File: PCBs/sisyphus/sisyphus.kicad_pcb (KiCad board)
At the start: 2 copper layers, 60 x 39.5 mm, 65 parts, among them J1 USB_C_Receptacle_USB2.0_14P, J2 AUX USB, J3 Conn_01x02, J4 Speaker, J5 SWD, J6 RGB_CONN, J7 Keyboard, J8 Light sensor, J9 Battery, U1 NCP1117-3.3_SOT223, U2 USBLC6-2P6, U3 W25Q128JVS, U4 MAX98357A, U5 RP2040, U7 BQ25619, Y1 ABM8-272-T3

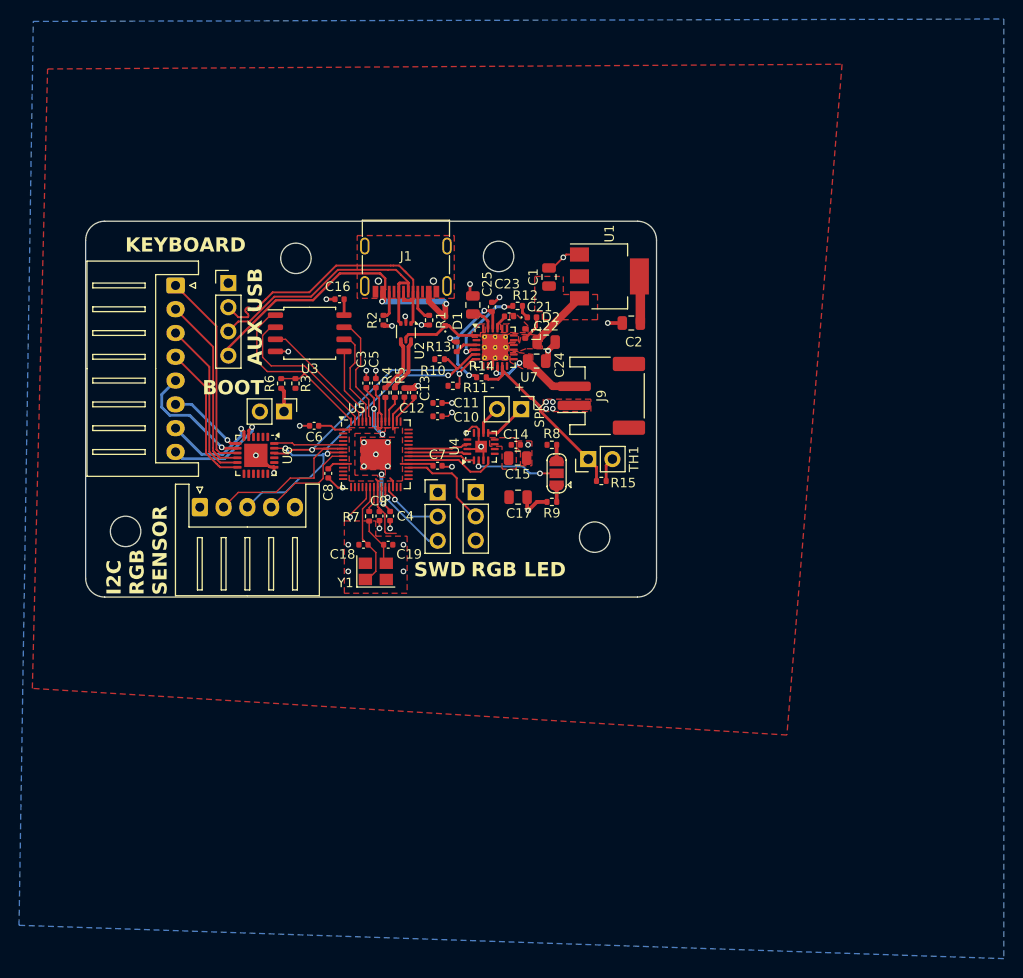
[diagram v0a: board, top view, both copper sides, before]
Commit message: Major PCB update
I won't even bother commenting it
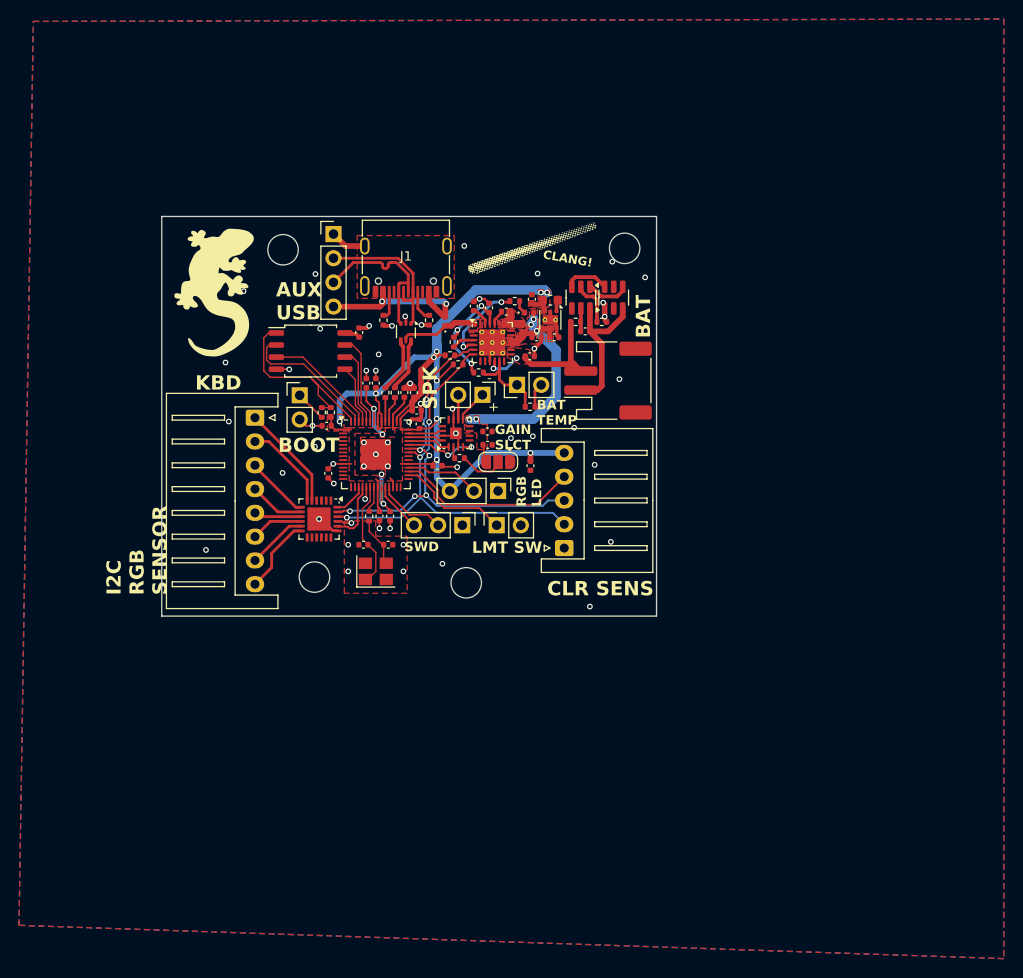
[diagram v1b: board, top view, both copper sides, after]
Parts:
- removed C1, C2: 10uF, Capacitor_SMD:C_0805_2012Metric
- removed R9: DNF, Resistor_SMD:R_0402_1005Metric
- removed U1: NCP1117-3.3_SOT223, Package_TO_SOT_SMD:SOT-223-3_TabPin2
- added C20: 100nF, Capacitor_SMD:C_0402_1005Metric, F.Cu at (122.0, 87.1)
- added C26: 10uF, Capacitor_SMD:C_0402_1005Metric, F.Cu at (116.4, 83.7)
- added C27: 10uF, Capacitor_SMD:C_0402_1005Metric, F.Cu at (118.8, 87.7)
- added J10: Limit SW, Connector_PinSocket_2.54mm:PinSocket_1x02_P2.54mm_Vertical, F.Cu at (112.7, 107.5)
- added L7: 2.2uH 1A, Inductor_SMD:L_0603_1608Metric, F.Cu at (118.3, 83.8)
- added Q1: FS8205, Package_TO_SOT_SMD:SOT-23-6, F.Cu at (125.0, 83.5)
- added R16: 100, Resistor_SMD:R_0402_1005Metric, F.Cu at (121.0, 86.1)
- added R17: 1k, Resistor_SMD:R_0402_1005Metric, F.Cu at (123.8, 86.1)
- added U10: TPS62293, Package_SON:WSON-6-1EP_2x2mm_P0.65mm_EP1x1.6mm_ThermalVias, F.Cu at (118.3, 85.9)
- added U8: DW01A, Package_TO_SOT_SMD:SOT-23-6, F.Cu at (121.5, 83.5)
- C15, C17, C22, C24, C25: footprint Capacitor_SMD:C_0805_2012Metric -> Capacitor_SMD:C_0402_1005Metric
- moved H3 38.9 mm to (93.5, 112.9)
- moved J8 38.5 mm to (119.8, 109.8), turned to 90 degrees
- moved H2 38.5 mm to (109.5, 113.5)
- moved H1 33.9 mm to (90.2, 78.5)
- moved H4 30.5 mm to (126.2, 78.3)
- moved J7 16.2 mm to (87.3, 96.2)
- moved J2 12.2 mm to (95.5, 76.8)
- moved R15 10.8 mm to (116.2, 95.0)
- moved TH1 10.8 mm to (114.8, 92.7)
- moved R8 9.80 mm to (108.8, 100.4)
- moved U6 9.43 mm to (94.0, 106.8)
- moved JP2 6.27 mm to (112.8, 100.8), turned to 180 degrees
- moved R6 5.25 mm to (94.3, 95.6)
- moved R3 4.81 mm to (95.3, 95.6)
- moved J4 4.34 mm to (111.2, 93.8)
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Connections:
- C14 pad 2: +3V3 -> VSYS
- C15 pad 2: +3V3 -> VSYS
- J7 pad 1: /COL0 -> /ROW3
- J7 pad 2: /COL1 -> /ROW2
- J7 pad 3: /COL2 -> /ROW1
- J7 pad 4: /COL3 -> /ROW0
- J7 pad 5: /ROW0 -> /COL0
- J7 pad 6: /ROW1 -> /COL1
- J7 pad 7: /ROW2 -> /COL2
- J7 pad 8: /ROW3 -> /COL3
- J9 pad 1: GND -> /B-
- JP2 pad 1: Net-(JP2-A) -> GND
- JP2 pad 2: /GAIN_SELECT -> Net-(JP2-C)
- JP2 pad 3: Net-(JP2-B) -> VSYS
- R8 pad 1: +3V3 -> /GAIN_SELECT
- R8 pad 2: Net-(JP2-B) -> Net-(JP2-C)
- U4 pad 7: +3V3 -> VSYS
- U4 pad 8: +3V3 -> VSYS
- U5 pad 17: unconnected-(U5-GPIO14-Pad17) -> /KEYPAD_INT
- U5 pad 18: unconnected-(U5-GPIO15-Pad18) -> /KEYPAD_RESET
- U5 pad 30: unconnected-(U5-GPIO19-Pad30) -> /LMT_SW
- U5 pad 31: unconnected-(U5-GPIO20-Pad31) -> /AUX_LED
- U5 pad 34: /I2S_ENABLE -> unconnected-(U5-GPIO22-Pad34)
- U5 pad 35: /I2S_DATA -> unconnected-(U5-GPIO23-Pad35)
- U5 pad 36: /I2S_BIT_CLOCK -> /SDA
- U5 pad 37: /I2S_FRAME_CLOCK -> /SCL
- U5 pad 38: unconnected-(U5-GPIO26_ADC0-Pad38) -> /I2S_ENABLE
- U5 pad 39: unconnected-(U5-GPIO27_ADC1-Pad39) -> /I2S_DATA
- U5 pad 40: unconnected-(U5-GPIO28_ADC2-Pad40) -> /I2S_BIT_CLOCK
- U5 pad 41: unconnected-(U5-GPIO29_ADC3-Pad41) -> /I2S_FRAME_CLOCK
- U5 pad 5: /KEYPAD_INT -> unconnected-(U5-GPIO3-Pad5)
- U5 pad 6: /SDA -> unconnected-(U5-GPIO4-Pad6)
- U5 pad 7: /SCL -> unconnected-(U5-GPIO5-Pad7)
- U5 pad 8: /AUX_LED -> unconnected-(U5-GPIO6-Pad8)
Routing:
- net +3V3: track 35.1 -> 111.7 mm, vias 0 -> 12
- net VSYS: track 9.12 -> 30.4 mm, vias 0 -> 5
- net /COL0: track 21.4 -> 4.96 mm
- net /B-: track 0.00 -> 16.0 mm
- net VBUS: track 35.0 -> 19.3 mm
- net /DN: track 30.5 -> 16.4 mm
- net /COL1: track 19.4 -> 5.46 mm
- net /DP: track 29.3 -> 17.1 mm
- net /LMT_SW: track 0.00 -> 11.8 mm
- net /COL2: track 17.4 -> 6.29 mm
- net Net-(U7-TS): track 19.2 -> 8.61 mm
- net /AUX_LED: track 10.6 -> 19.5 mm
- net /GAIN_SELECT: track 9.16 -> 1.23 mm, vias 2 -> 0
- net /COL3: track 15.4 -> 7.99 mm
- net /ROW0: track 13.1 -> 5.79 mm, vias 1 -> 0
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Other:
- board size 60 x 39.5 mm -> 52 x 42 mm
- board text added: "BAT"
- board text added: "BAT TEMP"
- board text added: "CLANG!"
- board text added: "CLR SENS"
- board text added: "GAIN SLCT"
- board text added: "KBD"
- board text added: "LMT SW"
- board text added: "Made with by Plajta"
- board text added: "Sisyfoss"
- board text added: "β"
- board text removed: "KEYBOARD"
- board text removed: "Made by Plajta"
- board text removed: "Sisyphus v0.1"
